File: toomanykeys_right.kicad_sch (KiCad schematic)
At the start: 81 parts, among them U1 TLV61070ADBV, U2 SN74LV1T126DBVR

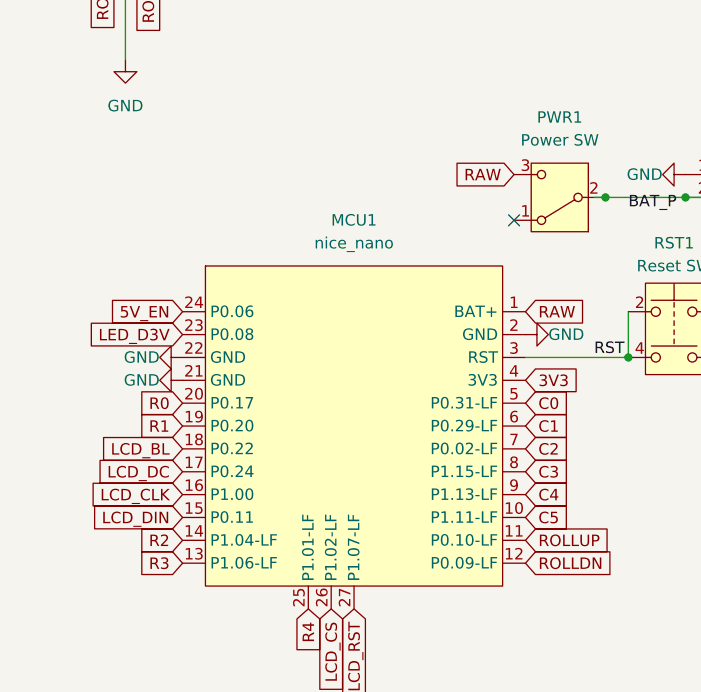
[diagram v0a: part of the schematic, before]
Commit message: Fully route left half. Schematic and PCB both clean!
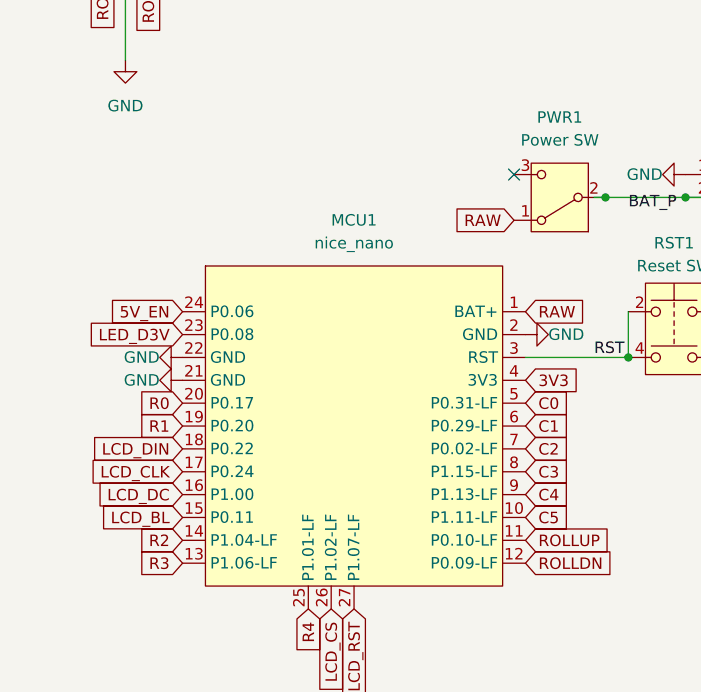
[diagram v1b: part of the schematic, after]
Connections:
- net LCD_BL: now also MCU1.15 (P0.11); no longer MCU1.18 (P0.22)
- net LCD_CLK: now also MCU1.17 (P0.24); no longer MCU1.16 (P1.00)
- net LCD_DC: now also MCU1.16 (P1.00); no longer MCU1.17 (P0.24)
- net LCD_DIN: now also MCU1.18 (P0.22); no longer MCU1.15 (P0.11)
- net RAW: now also PWR1.1 (A); no longer PWR1.3 (C)
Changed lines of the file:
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@@
 	)
 	(no_connect
-		(at 69.85 137.16)
+		(at 69.85 132.08)
 	)
 	(wire
@@
 		)
 	)
-	(global_label "LCD_CLK"
+	(global_label "R0"
 		(shape input)
-		(at 33.02 167.64 180)
+		(at 33.02 157.48 180)
 		(fields_autoplaced yes)
 		(effects
@@
 		)
 		(property "Intersheetrefs" "${INTERSHEET_REFS}"
-			(at 21.931 167.64 0)
+			(at 27.5553 157.48 0)
 			(effects
 				(font
@@
 		)
 	)
-	(global_label "R0"
+	(global_label "LCD_CLK"
 		(shape input)
-		(at 33.02 157.48 180)
+		(at 33.02 165.1 180)
 		(fields_autoplaced yes)
 		(effects
@@
 		)
 		(property "Intersheetrefs" "${INTERSHEET_REFS}"
-			(at 27.5553 157.48 0)
+			(at 21.931 165.1 0)
 			(effects
 				(font
@@
 	(global_label "LCD_BL"
 		(shape input)
-		(at 137.16 158.75 90)
+		(at 33.02 170.18 180)
 		(fields_autoplaced yes)
 		(effects
@@
 				(size 1.27 1.27)
 			)
-			(justify left)
+			(justify right)
 		)
 		(property "Intersheetrefs" "${INTERSHEET_REFS}"
-			(at 137.16 148.931 90)
+			(at 23.201 170.18 0)
 			(effects
 				(font
 					(size 1.27 1.27)
 				)
-				(justify left)
+				(justify right)
 				(hide yes)
 			)
 		)
 	)
-	(global_label "C2"
+	(global_label "LCD_BL"
 		(shape input)
-		(at 99.06 21.59 90)
+		(at 137.16 158.75 90)
 		(fields_autoplaced yes)
 		(effects
@@
 		)
 		(property "Intersheetrefs" "${INTERSHEET_REFS}"
-			(at 99.06 16.1253 90)
+			(at 137.16 148.931 90)
 			(effects
 				(font
@@
 		)
 	)
-	(global_label "R1"
+	(global_label "C2"
 		(shape input)
-		(at 38.1 48.26 180)
+		(at 99.06 21.59 90)
 		(fields_autoplaced yes)
 		(effects
@@
 				(size 1.27 1.27)
 			)
-			(justify right)
+			(justify left)
 		)
 		(property "Intersheetrefs" "${INTERSHEET_REFS}"
-			(at 32.6353 48.26 0)
+			(at 99.06 16.1253 90)
 			(effects
 				(font
 					(size 1.27 1.27)
 				)
-				(justify right)
+				(justify left)
 				(hide yes)
 			)
 		)
 	)
-	(global_label "LCD_BL"
+	(global_label "R1"
 		(shape input)
-		(at 33.02 162.56 180)
+		(at 38.1 48.26 180)
 		(fields_autoplaced yes)
 		(effects
@@
 		)
 		(property "Intersheetrefs" "${INTERSHEET_REFS}"
-			(at 23.201 162.56 0)
+			(at 32.6353 48.26 0)
 			(effects
 				(font
@@
 		)
 	)
-	(global_label "LCD_DC"
-		(shape input)
-		(at 33.02 165.1 180)
-		(fields_autoplaced yes)
-		(effects
-			(font
-				(size 1.27 1.27)
-			)
-			(justify right)
-		)
-		(property "Intersheetrefs" "${INTERSHEET_REFS}"
-			(at 22.9591 165.1 0)
-			(effects
-				(font
-					(size 1.27 1.27)
-				)
-				(justify right)
-				(hide yes)
-			)
-		)
-	)
 	(global_label "RAW"
 		(shape input)
@@
 		)
 	)
+	(global_label "RAW"
+		(shape input)
+		(at 69.85 137.16 180)
+		(fields_autoplaced yes)
+		(effects
+			(font
+				(size 1.27 1.27)
+			)
+			(justify right)
+		)
+		(property "Intersheetrefs" "${INTERSHEET_REFS}"
+			(at 63.0548 137.16 0)
+			(effects
+				(font
+					(size 1.27 1.27)
+				)
+				(justify right)
+				(hide yes)
+			)
+		)
+	)
 	(global_label "R2"
 		(shape input)
@@
 		)
 	)
+	(global_label "LCD_DC"
+		(shape input)
+		(at 33.02 167.64 180)
+		(fields_autoplaced yes)
+		(effects
+			(font
+				(size 1.27 1.27)
+			)
+			(justify right)
+		)
+		(property "Intersheetrefs" "${INTERSHEET_REFS}"
+			(at 22.9591 167.64 0)
+			(effects
+				(font
+					(size 1.27 1.27)
+				)
+				(justify right)
+				(hide yes)
+			)
+		)
+	)
 	(global_label "C1"
 		(shape input)
@@
 	(global_label "LCD_DIN"
 		(shape input)
-		(at 33.02 170.18 180)
-		(fields_autoplaced yes)
-		(effects
-			(font
-				(size 1.27 1.27)
-			)
-			(justify right)
-		)
-		(property "Intersheetrefs" "${INTERSHEET_REFS}"
-			(at 22.2938 170.18 0)
-			(effects
-				(font
-					(size 1.27 1.27)
-				)
-				(justify right)
-				(hide yes)
-			)
-		)
-	)
-	(global_label "RAW"
-		(shape input)
-		(at 69.85 132.08 180)
+		(at 33.02 162.56 180)
 		(fields_autoplaced yes)
 		(effects
@@
 		)
 		(property "Intersheetrefs" "${INTERSHEET_REFS}"
-			(at 63.0548 132.08 0)
+			(at 22.2938 162.56 0)
 			(effects
 				(font
